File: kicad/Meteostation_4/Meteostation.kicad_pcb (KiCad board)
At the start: 2 copper layers, 44 x 44 mm, 106 parts, among them J1 TxD, J10 GM+, J11 GM-, J12 SWD, J13 SWC, J2 RxD, J3 BME280_SCL, J4 BME280_SDA, J6 +EXT, J7 -EXT, Q1 5N10, Q2 IRLML6346, Q3 Q_NPN_BEC, T1 HY931147C, U1 STM32F103C8Tx, U2 LMR14206, U3 AD8541, Y2 ECS-250-20-33 25MHz

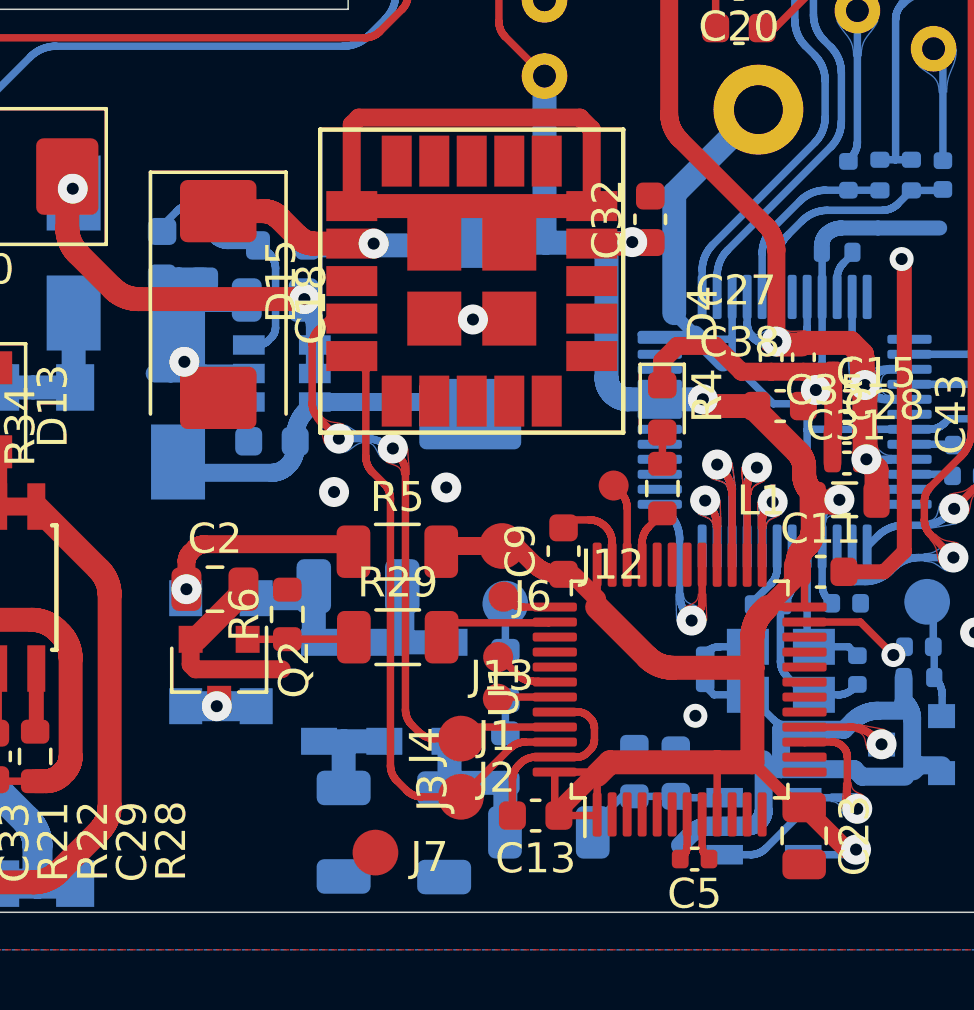
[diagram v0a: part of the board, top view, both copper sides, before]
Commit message: изменено:      kicad/Meteostation_4/Meteostation.kicad_pcb 	изменено:      kicad/Meteostation_4/Meteostation.kicad_pcb-bak 	изменено:      kicad/Meteostation_4/Meteostation.sch 	изменено:      kicad/Meteostation_4/Meteostation.sch-bak 	изменено:      kicad/Meteostation_4/fp-info-cache 	изменено:      kicad/Meteostation_4/gerber/Meteostation-job.gbrjob
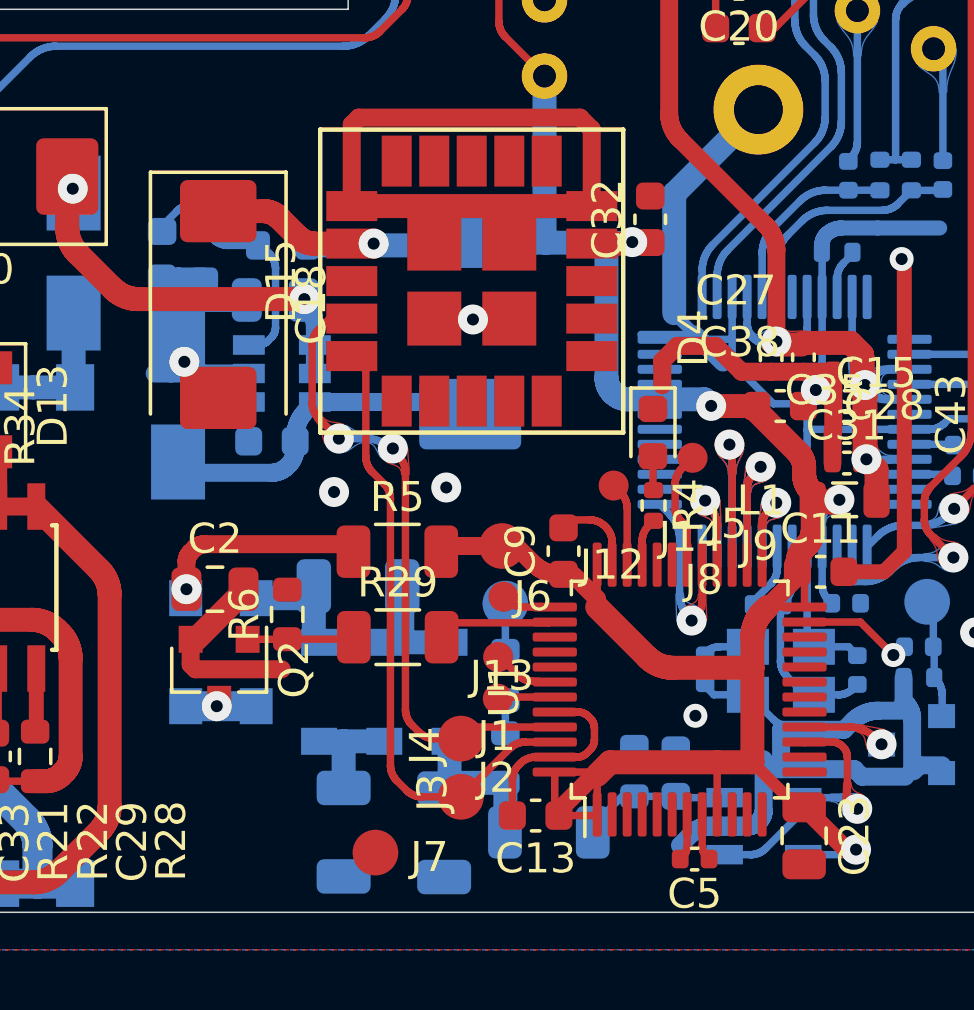
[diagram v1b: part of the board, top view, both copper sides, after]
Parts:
- added J14: DISP_CS, My-library:ConnMini, F.Cu at (53.0, 89.2)
- added J5: miso, My-library:ConnMini, F.Cu at (54.2, 88.8)
- added J8: mosi, My-library:ConnMini, F.Cu at (53.4, 90.7)
- added J9: sclk, My-library:ConnMini, F.Cu at (55.2, 89.5)
- R4: footprint Resistor_SMD:R_0603_1608Metric -> Resistor_SMD:R_0402_1005Metric
- moved D4 0.85 mm to (51.7, 88.4)
- moved R4 0.64 mm to (51.7, 90.8)
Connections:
- U1 pad 30: (no net) -> Net-(J14-Pad1)
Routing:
- net Net-(J14-Pad1): track 0.00 -> 3.90 mm
- net MISO: track 6.47 -> 7.56 mm
